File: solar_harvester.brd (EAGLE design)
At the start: 46 x 25.4 mm, 44 parts, among them U1 BQ25505, U2 TPS61322XA, U3 TPS61322XA, U4 MAX17040, U5 INA226, U6 DMP3085LSD

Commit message: BOM updated
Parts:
- R3: value 7.32M -> 1.2M
- R4: value 7.32M -> 7.5M
- R5: value 7.32M -> 4.3M
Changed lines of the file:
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@@
 <attribute name="NAME" x="15.6436" y="14.1744" size="0.6096" layer="25"/>
 </element>
-<element name="R3" library="vrlib_res" package="RESISTOR_1608_FOOTPRINT" value="7.32M" x="13.2574" y="12.7762" smashed="yes" rot="R270">
+<element name="R3" library="vrlib_res" package="RESISTOR_1608_FOOTPRINT" value="1.2M" x="13.2574" y="12.7762" smashed="yes" rot="R270">
 <attribute name="NAME" x="11.763" y="13.2226" size="0.6096" layer="25" rot="R180"/>
 </element>
-<element name="R4" library="vrlib_res" package="RESISTOR_1608_FOOTPRINT" value="7.32M" x="17.4752" y="7.8822" smashed="yes">
+<element name="R4" library="vrlib_res" package="RESISTOR_1608_FOOTPRINT" value="7.5M" x="17.4752" y="7.8822" smashed="yes">
 <attribute name="NAME" x="16.4874" y="8.8696" size="0.6096" layer="25" rot="R180"/>
 </element>
-<element name="R5" library="vrlib_res" package="RESISTOR_1608_FOOTPRINT" value="7.32M" x="20.1752" y="7.239" smashed="yes" rot="R90">
+<element name="R5" library="vrlib_res" package="RESISTOR_1608_FOOTPRINT" value="4.3M" x="20.1752" y="7.239" smashed="yes" rot="R90">
 <attribute name="NAME" x="21.7396" y="6.888" size="0.6096" layer="25"/>
 </element>

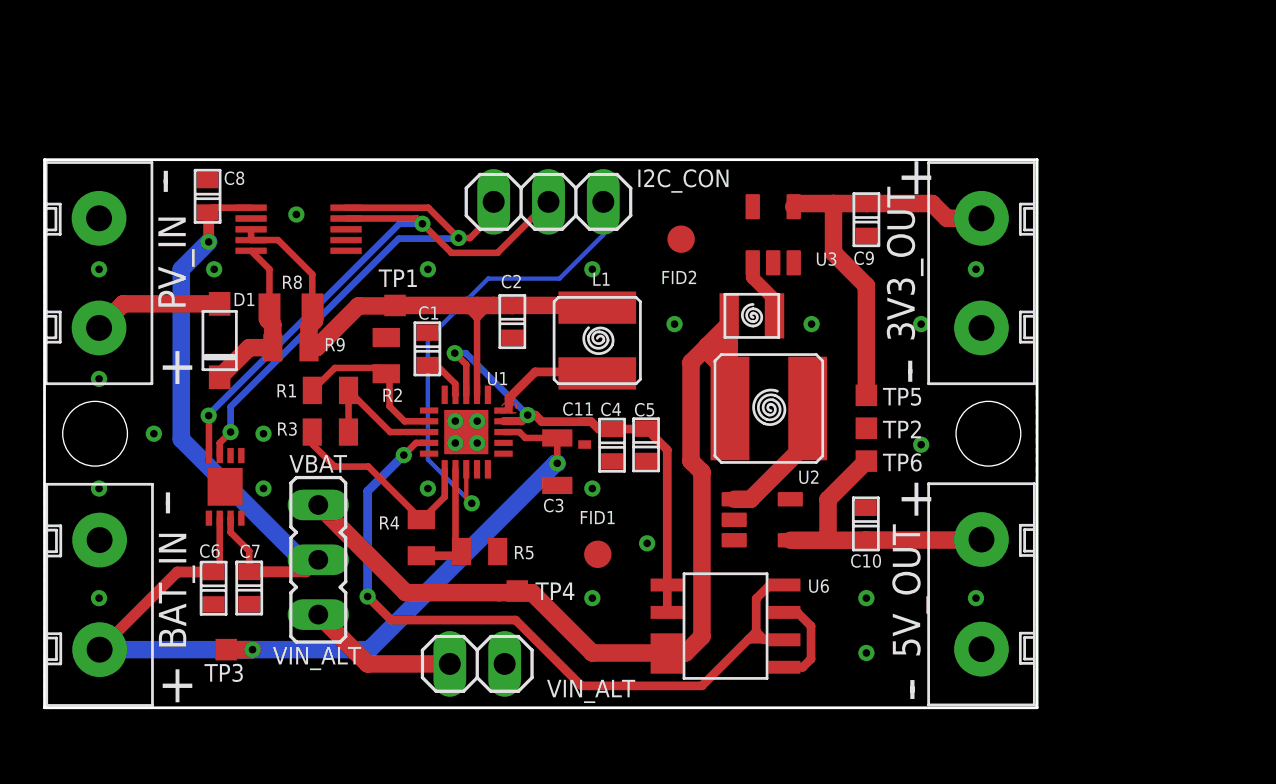
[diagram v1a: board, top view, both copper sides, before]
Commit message: Rev2
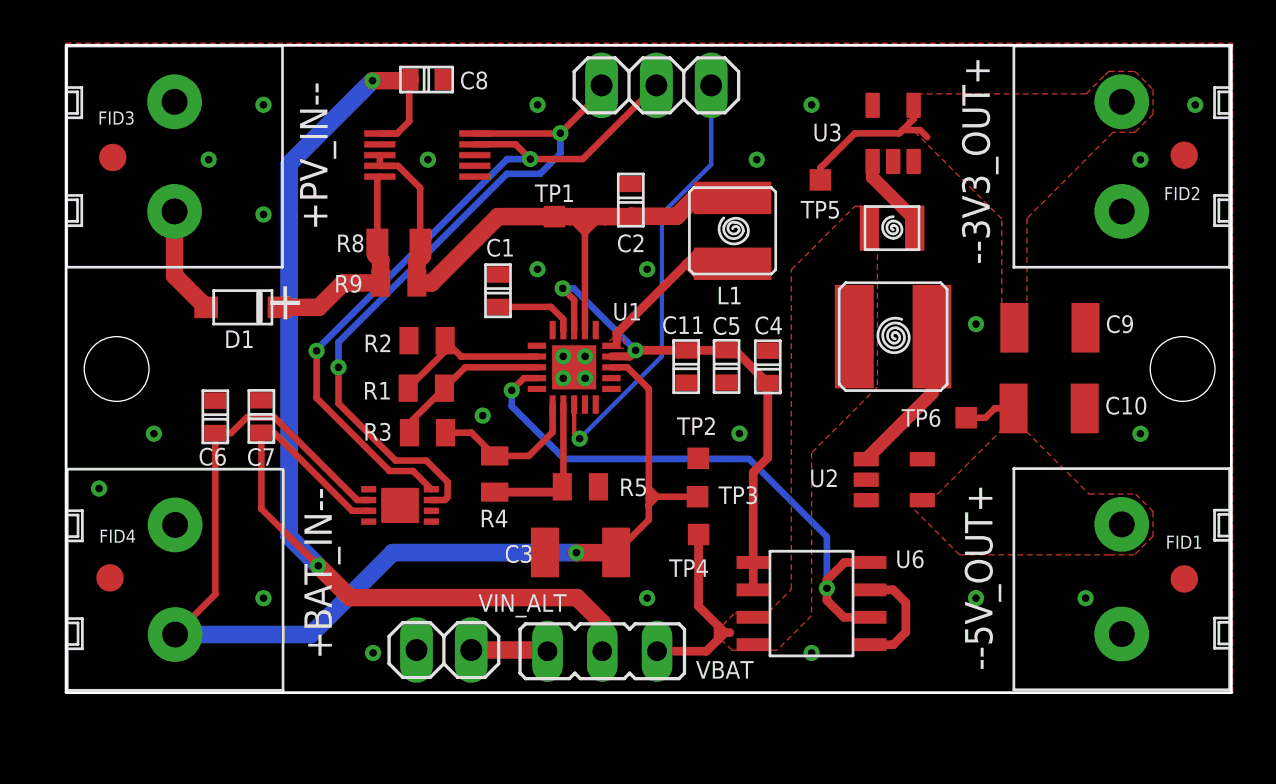
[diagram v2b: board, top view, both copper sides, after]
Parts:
- removed 3V3_OUT, 5V_OUT, BAT_IN, PV_IN: CONN_SCEW_TYPE_2P, vrlib_connector:CONN_SCREW_TYPE_2P
- added +BAT_IN--, +PV_IN--, --3V3_OUT+, --5V_OUT+: CONN_SCEW_TYPE_2P, vrlib_connector:CONN_SCREW_TYPE_2P
- added FID3, FID4: FIDUCIAL_25, vrlib_prod:FIDUCIAL_25
- C10, C9: value 22u -> 100u; device vrlib_caps:1608_FOOTPRINT -> vrlib_caps:3528_TAN_FOOTPRINT
- C11: device vrlib_caps:1005_FOOTPRINT -> vrlib_caps:1608_FOOTPRINT
- C3: device vrlib_caps:2012_FOOTPRINT -> vrlib_caps:3528_TAN_FOOTPRINT
- moved FID1 27.2 mm to (52.8, 5.97)
- moved FID2 23.6 mm to (52.8, 25.6)
- moved TP3 23.0 mm to (30.3, 9.78)
- moved JP4 13.8 mm to (25.9, 2.62), turned to 180 degrees
- moved C8 11.5 mm to (17.7, 29.1), turned to 90 degrees
- moved TP5 10.2 mm to (36.0, 24.5)
- moved C10 10.0 mm to (46.6, 13.9), turned to 270 degrees
- moved C9 9.87 mm to (46.6, 17.6), turned to 270 degrees
- moved TP4 8.80 mm to (30.3, 8.03)
- moved TP1 8.46 mm to (23.6, 22.8)
- moved U4 8.15 mm to (16.5, 9.38), turned to 270 degrees
- moved C4 8.08 mm to (33.5, 15.8), turned to 180 degrees
- moved L1 8.07 mm to (31.9, 22.1)
- moved C7 7.97 mm to (10.1, 13.5), turned to 180 degrees
- moved C6 7.94 mm to (7.93, 13.5), turned to 180 degrees
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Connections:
- net GND: now also +BAT_IN--.2, +PV_IN--.2, --3V3_OUT+.2, --5V_OUT+.2; no longer 3V3_OUT.2, 5V_OUT.2, BAT_IN.2, PV_IN.2
- net N$7: now also +PV_IN--.1; no longer PV_IN.1
- net VDD3V3: now also --3V3_OUT+.1; no longer 3V3_OUT.1
- net VDD5: now also --5V_OUT+.1; no longer 5V_OUT.1
- net VIN_BAT: now also +BAT_IN--.1; no longer BAT_IN.1
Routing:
- net VCC: track 45.5 -> 10.2 mm
- net VCC_MIX: track 28.1 -> 59.2 mm, vias 1 -> 2
- net VIN_BAT: track 39.2 -> 54.9 mm, vias 2 -> 1
- net VDD5: track 13.3 -> 2.38 mm
- net VDD3V3: track 18.6 -> 7.73 mm
- net I2C_SCL: track 24.7 -> 32.8 mm
- net !VB_SEC_ON!: track 35.1 -> 27.2 mm
- net I2C_SDA: track 26.5 -> 33.0 mm
- net N$1: track 5.31 -> 9.09 mm
- net VIN_ALT: track 7.04 -> 3.55 mm
- net PVIN_AN: track 27.8 -> 31.2 mm
- net N$5: track 9.86 -> 7.14 mm
- net PVIN: track 8.00 -> 10.3 mm
- net VCC_P: track 22.6 -> 24.6 mm
- net N$2: track 2.17 -> 3.77 mm
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- added copper zone on layer 1, net VCC
- added copper zone on layer 1, net VDD3V3
- added copper zone on layer 1, net VDD5
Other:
- board size 46 x 25.4 mm -> 54 x 30 mm
- board text added: "Rev 2"
- board text removed: "-"
- board text removed: "I2C_CON"
- board text removed: "Rev 1"
